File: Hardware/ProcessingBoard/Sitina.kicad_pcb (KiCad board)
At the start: 4 copper layers, 100 x 68 mm, 134 parts, among them J1 Conn_01x30_MountingPin, J200 Conn_02x05_Odd_Even, J500 USB_B_Micro, J700 TXW280064B0, Q400 2N7002, SW200 SW_DIP_x02, SW600 SW_Push, SW601 SW_Push, SW602 SW_Push, SW603 SW_Push, SW610 SW_Push, SW611 SW_Push, SW612 TM-4175-B-B, U100 IMXRT1050, U300 MT48LC16M16A2BG, U400 ADP163, U401 W25Q32JVZP, U500 USBLC6-2SC6, U700 CAT4139, U9 LTC3567, Y100 24MHz, Y101 32.768K

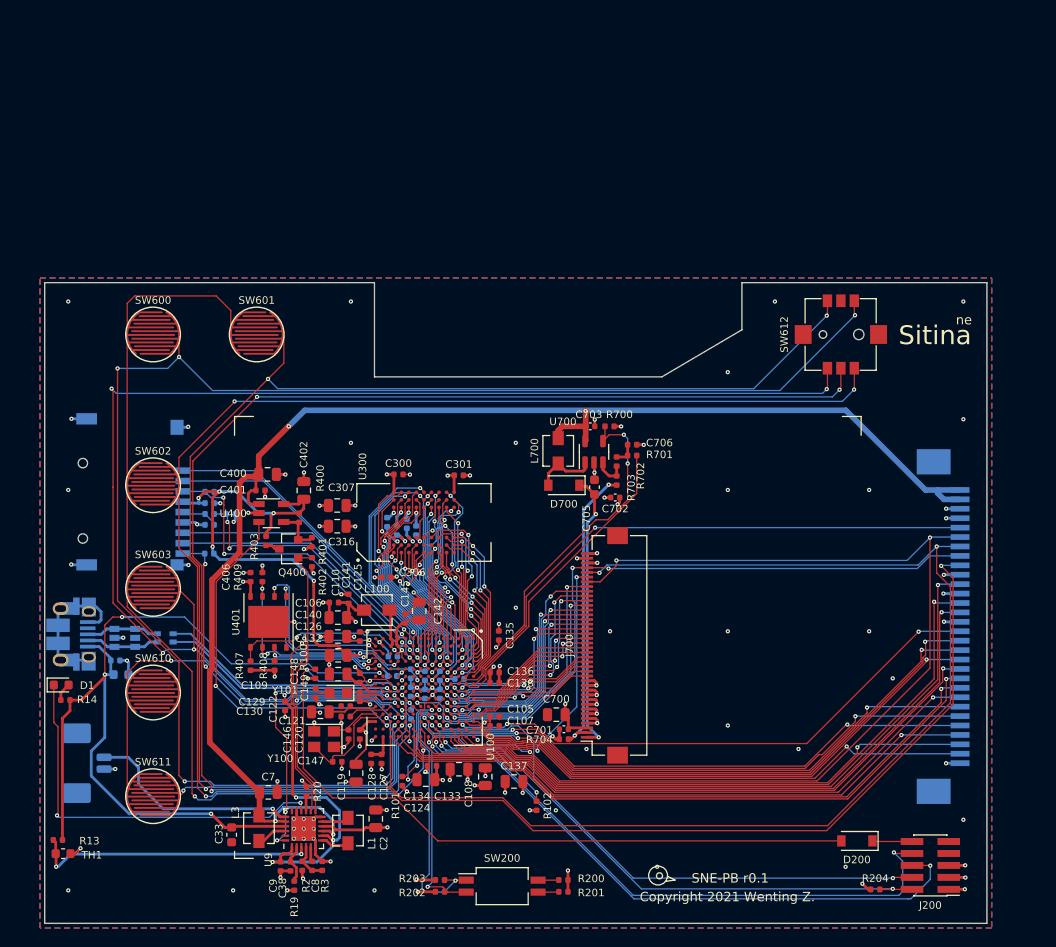
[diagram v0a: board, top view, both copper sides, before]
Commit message: Bug fixes and changes for PB r0p2
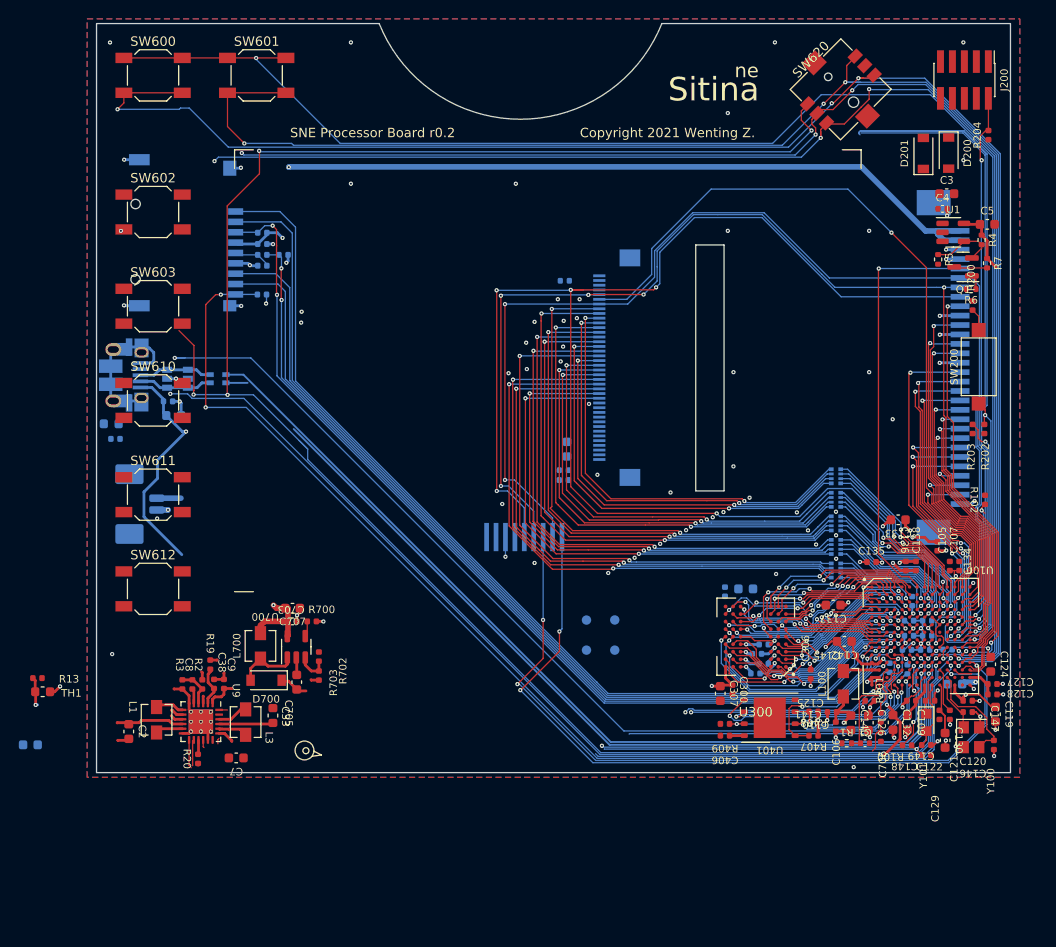
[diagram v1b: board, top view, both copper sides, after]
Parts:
- removed C400: 10uF, Capacitor_SMD:C_0805_2012Metric
- removed C401: 100nF, Capacitor_SMD:C_0402_1005Metric
- removed Q400: 2N7002, Package_TO_SOT_SMD:SOT-23
- removed R101: 10K, Resistor_SMD:R_0402_1005Metric
- removed R201: 1K, Resistor_SMD:R_0402_1005Metric
- removed R400: 464K/1%, Resistor_SMD:R_0402_1005Metric
- removed R401, R402: 200K/1%, Resistor_SMD:R_0402_1005Metric
- removed R403: 243K/1%, Resistor_SMD:R_0402_1005Metric
- removed U400: ADP163, Package_TO_SOT_SMD:TSOT-23-5
- added C1: 0.22uF, Capacitor_SMD:C_0402_1005Metric, F.Cu at (169.6, 139.4)
- added C3: 10uF, Capacitor_SMD:C_0603_1608Metric, F.Cu at (178.2, 81.1)
- added C4: 100nF, Capacitor_SMD:C_0402_1005Metric, F.Cu at (177.8, 82.7)
- added C5: 10uF, Capacitor_SMD:C_0603_1608Metric, F.Cu at (182.5, 84.3)
- added C707: 10uF, Capacitor_SMD:C_0603_1608Metric, F.Cu at (108.8, 125.0)
- added D201: 1N5819, Diode_SMD:D_SOD-123, F.Cu at (175.8, 76.8)
- added J701: Conn_01x09, Footprints:FPC_9, B.Cu at (133.4, 117.5)
- added Q1: 2N7002, Package_TO_SOT_SMD:SOT-23, F.Cu at (180.0, 88.8)
- added R1: 30K, Resistor_SMD:R_0402_1005Metric, F.Cu at (167.6, 139.4)
- added R4: 464K/1%, Resistor_SMD:R_0402_1005Metric, F.Cu at (181.9, 86.0)
- added R5: 200K/1%, Resistor_SMD:R_0402_1005Metric, F.Cu at (177.3, 88.0)
- added R6: 200K/1%, Resistor_SMD:R_0402_1005Metric, F.Cu at (180.8, 91.2)
- added R7: 243K/1%, Resistor_SMD:R_0402_1005Metric, F.Cu at (182.5, 88.4)
- added RN700: 33R, Resistor_SMD:R_Array_Convex_4x0402, B.Cu at (166.5, 111.0)
- added RN701: 33R, Resistor_SMD:R_Array_Convex_4x0402, B.Cu at (166.5, 113.5)
- added RN702: 33R, Resistor_SMD:R_Array_Convex_4x0402, B.Cu at (166.5, 116.0)
- added RN703: 33R, Resistor_SMD:R_Array_Convex_4x0402, B.Cu at (166.5, 118.5)
- added RN704: 33R, Resistor_SMD:R_Array_Convex_4x0402, B.Cu at (166.5, 121.0)
- added SW620: TM-4175-B-B, Footprints:TM4175, F.Cu at (167.0, 70.0)
- added TP1: TestPoint_Small, TestPoint:TestPoint_Pad_D1.0mm, B.Cu at (140.0, 126.3)
- added TP2: TestPoint_Small, TestPoint:TestPoint_Pad_D1.0mm, B.Cu at (140.0, 129.5)
- added TP3: TestPoint_Small, TestPoint:TestPoint_Pad_D1.0mm, B.Cu at (143.0, 126.3)
- added TP4: TestPoint_Small, TestPoint:TestPoint_Pad_D1.0mm, B.Cu at (143.0, 129.5)
- added U1: ADP163, Package_TO_SOT_SMD:TSOT-23-5, F.Cu at (178.9, 85.2)
- C108, C316, C402, C700: footprint Capacitor_SMD:C_0805_2012Metric -> Capacitor_SMD:C_0603_1608Metric; moved to B.Cu
- C109, C119, C124, C126, C130, C132, C133, C137, C140, C142, C2, C307, C7: footprint Capacitor_SMD:C_0805_2012Metric -> Capacitor_SMD:C_0603_1608Metric
- C301, C701, C702, D1, R14, R704: moved to B.Cu
- C404, C405: value 18pF -> DNP
- J700: value TXW280064B0 -> TXW280064B0-R; moved to B.Cu
- L700: value 2.2uH -> 22uH
- SW200: value SW_DIP_x02 -> DNP; footprint Button_Switch_SMD:SW_DIP_SPSTx02_Slide_Copal_CHS-02B_W7.62mm_P1.27mm -> Button_Switch_SMD:SW_SPST_CK_RS282G05A3
- SW600, SW601, SW602, SW603, SW610, SW611: footprint Footprints:contact -> Button_Switch_SMD:SW_SPST_SKQG_WithStem
- SW612: value TM-4175-B-B -> SW_Push; footprint Footprints:TM4175 -> Button_Switch_SMD:SW_SPST_SKQG_WithStem
- U300: footprint Footprints:BGA-54_9x9_8.0x14.0mm -> Footprints:BGA-54_9x9_8.0x8.0mm
- moved J200 83.4 mm to (180.1, 69.0), turned to -90 degrees
- moved R204 81.0 mm to (182.7, 74.8), turned to 90 degrees
- moved SW612 77.8 mm to (94.0, 123.0), turned to 0 degrees
- moved R202 75.8 mm to (182.2, 106.0), turned to -90 degrees
- moved R200 74.9 mm to (181.0, 92.9), turned to 90 degrees
- moved SW200 74.8 mm to (181.6, 99.4), turned to 90 degrees
- moved R203 74.1 mm to (181.0, 106.0), turned to -90 degrees
- moved D200 73.6 mm to (178.4, 76.8), turned to -90 degrees
- moved C147 69.7 mm to (183.2, 139.6), turned to -90 degrees
- moved Y100 68.7 mm to (180.9, 138.8), turned to -90 degrees
- moved C122 68.3 mm to (176.1, 140.6), turned to 0 degrees
- moved C119 68.1 mm to (183.4, 136.3)
- moved C130 66.4 mm to (178.1, 139.1), turned to -90 degrees
- moved C128 66.3 mm to (183.1, 134.2), turned to 0 degrees
- moved C146 65.8 mm to (180.5, 136.1), turned to 0 degrees
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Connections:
- net /MCU/AFE_SYNC renamed /cb_interface/AFE_SYNC
- net /MCU/CSI_D0 renamed /cb_interface/CSI_D0
- net /MCU/CSI_D1 renamed /cb_interface/CSI_D1
- net /MCU/CSI_D10 renamed /cb_interface/CSI_D10
- net /MCU/CSI_D11 renamed /cb_interface/CSI_D11
- net /MCU/CSI_D12 renamed /cb_interface/CSI_D12
- net /MCU/CSI_D13 renamed /cb_interface/CSI_D13
- net /MCU/CSI_D2 renamed /cb_interface/CSI_D2
- net /MCU/CSI_D3 renamed /cb_interface/CSI_D3
- net /MCU/CSI_D4 renamed /cb_interface/CSI_D4
- net /MCU/CSI_D5 renamed /cb_interface/CSI_D5
- net /MCU/CSI_D6 renamed /cb_interface/CSI_D6
- net /MCU/CSI_D7 renamed /cb_interface/CSI_D7
- net /MCU/CSI_D8 renamed /cb_interface/CSI_D8
- net /MCU/CSI_D9 renamed /cb_interface/CSI_D9
- net /MCU/CSI_HSYNC renamed /cb_interface/CSI_HSYNC
- net /MCU/CSI_PCLK renamed /cb_interface/CSI_PCLK
- net /MCU/CSI_VSYNC renamed /cb_interface/CSI_VSYNC
- net /MCU/JTAG_MOD renamed /mcu/JTAG_MOD
- net /MCU/JTAG_TCK renamed /debug/JTAG_TCK
- net /MCU/JTAG_TMS renamed /debug/JTAG_TMS
- net /MCU/KO0 renamed /key/KO0
- net /MCU/LCD_EN renamed /lcd/LCD_EN
- net /MCU/ON renamed /mcu/ON
- net /MCU/POR renamed /debug/SYS_RST
- net /MCU/QSPI_D0 renamed /mcu/QSPI_D0
- net /MCU/QSPI_D1 renamed /mcu/QSPI_D1
- net /MCU/QSPI_D2 renamed /mcu/QSPI_D2
- net /MCU/QSPI_D3 renamed /mcu/QSPI_D3
- net /MCU/QSPI_SCK renamed /mcu/QSPI_SCK
- net /MCU/QSPI_SS_B renamed /mcu/QSPI_SS_B
- net /MCU/SDRAM_A0 renamed /mcu/SDRAM_A0
- net /MCU/SDRAM_A1 renamed /mcu/SDRAM_A1
- net /MCU/SDRAM_A10 renamed /mcu/SDRAM_A10
- net /MCU/SDRAM_A11 renamed /mcu/SDRAM_A11
- net /MCU/SDRAM_A12 renamed /mcu/SDRAM_A12
- net /MCU/SDRAM_A2 renamed /mcu/SDRAM_A2
- net /MCU/SDRAM_A3 renamed /mcu/SDRAM_A3
- net /MCU/SDRAM_A4 renamed /mcu/SDRAM_A4
- net /MCU/SDRAM_A5 renamed /mcu/SDRAM_A5
- net /MCU/SDRAM_A6 renamed /mcu/SDRAM_A6
- net /MCU/SDRAM_A7 renamed /mcu/SDRAM_A7
- net /MCU/SDRAM_A8 renamed /mcu/SDRAM_A8
- net /MCU/SDRAM_A9 renamed /mcu/SDRAM_A9
- net /MCU/SDRAM_BA0 renamed /mcu/SDRAM_BA0
- net /MCU/SDRAM_BA1 renamed /mcu/SDRAM_BA1
- net /MCU/SDRAM_CKE renamed /sdram/SDRAM_CKE
- net /MCU/SDRAM_CLK renamed /sdram/SDRAM_CLK
- net /MCU/SDRAM_D0 renamed /mcu/SDRAM_D0
- net /MCU/SDRAM_D1 renamed /mcu/SDRAM_D1
- net /MCU/SDRAM_D10 renamed /mcu/SDRAM_D10
- net /MCU/SDRAM_D11 renamed /mcu/SDRAM_D11
- net /MCU/SDRAM_D12 renamed /mcu/SDRAM_D12
- net /MCU/SDRAM_D13 renamed /mcu/SDRAM_D13
- net /MCU/SDRAM_D14 renamed /mcu/SDRAM_D14
- net /MCU/SDRAM_D15 renamed /mcu/SDRAM_D15
- net /MCU/SDRAM_D2 renamed /mcu/SDRAM_D2
- net /MCU/SDRAM_D3 renamed /mcu/SDRAM_D3
- net /MCU/SDRAM_D4 renamed /mcu/SDRAM_D4
- net /MCU/SDRAM_D5 renamed /mcu/SDRAM_D5
- net /MCU/SDRAM_D6 renamed /mcu/SDRAM_D6
- net /MCU/SDRAM_D7 renamed /mcu/SDRAM_D7
- net /MCU/SDRAM_D8 renamed /mcu/SDRAM_D8
- net /MCU/SDRAM_D9 renamed /mcu/SDRAM_D9
- net /MCU/SDRAM_DM0 renamed /mcu/SDRAM_DM0
- net /MCU/SDRAM_DM1 renamed /mcu/SDRAM_DM1
- net /MCU/SD_CD_B renamed /mcu/SD_CD_B
- net /MCU/SD_CLK renamed /mcu/SD_CLK
- net /MCU/SD_D0 renamed /mcu/SD_D0
- net /MCU/SD_D1 renamed /mcu/SD_D1
- net /MCU/SD_D2 renamed /mcu/SD_D2
- net /MCU/SD_D3 renamed /mcu/SD_D3
- net /MCU/USB_DP renamed /mcu/USB_DP
- net /SDRAM/SDRAM_CAS renamed /sdram/SDRAM_CAS
- net /SDRAM/SDRAM_CS0 renamed /sdram/SDRAM_CS0
- net /SDRAM/SDRAM_RAS renamed /sdram/SDRAM_RAS
- net /SDRAM/SDRAM_WE renamed /sdram/SDRAM_WE
- net /storage/SD_CMD renamed /mcu/SD_CMD
- net /usb/USB_DM renamed /mcu/USB_DN
- C402 pad 1: +VSD -> +3V3
- C403 pad 1: +VSD -> +3V3
- J1 pad 22: /MCU/SPI_CS -> /cb_interface/AFE_SL
- J1 pad 23: /MCU/LCD_DI -> /cb_interface/AFE_SDATA
- J1 pad 24: /MCU/LCD_SCK -> /cb_interface/AFE_SCK
- J1 pad 25: /connector/AFE_RST -> /cb_interface/AFE_RST
- J200 pad 1: +3V3 -> Net-(D201-Pad2)
- J200 pad 6: /MCU/JTAG_TDO -> (no net)
- J200 pad 8: /MCU/JTAG_TDI -> (no net)
- J700 pad 1: /lcd/LEDA -> GND
- J700 pad 10: GND -> /lcd/D_D13
- J700 pad 11: GND -> /lcd/D_D12
- J700 pad 12: GND -> /lcd/D_D11
- J700 pad 13: GND -> /lcd/D_D10
- J700 pad 14: /MCU/LCD_VSYNC -> /lcd/D_D9
- J700 pad 15: /MCU/LCD_HSYNC -> /lcd/D_D8
- J700 pad 16: /MCU/LCD_CLK -> /lcd/D_D7
- J700 pad 17: /MCU/LCD_DE -> /lcd/D_D6
- J700 pad 18: /MCU/LCD_D0 -> /lcd/D_D5
- J700 pad 19: /MCU/LCD_D1 -> /lcd/D_D4
- J700 pad 2: /lcd/LEDK -> +3V3
- J700 pad 20: /MCU/LCD_D2 -> /lcd/D_D3
- J700 pad 21: /MCU/LCD_D3 -> /lcd/D_D2
- J700 pad 22: /MCU/LCD_D4 -> /lcd/D_D1
- J700 pad 23: /MCU/LCD_D5 -> /lcd/D_D0
- J700 pad 24: /MCU/LCD_D6 -> /lcd/D_DE
- J700 pad 25: /MCU/LCD_D7 -> /lcd/D_DCLK
- J700 pad 26: /MCU/LCD_D8 -> /lcd/D_HSYNC
- J700 pad 27: /MCU/LCD_D9 -> /lcd/D_VSYNC
- J700 pad 28: /MCU/LCD_D10 -> GND
- J700 pad 29: /MCU/LCD_D11 -> GND
- J700 pad 3: +3V3 -> GND
- J700 pad 30: /MCU/LCD_D12 -> GND
- J700 pad 31: /MCU/LCD_D13 -> GND
- J700 pad 32: /MCU/LCD_D14 -> GND
- J700 pad 33: /MCU/LCD_D15 -> GND
- J700 pad 34: /connector/AFE_RST -> GND
- J700 pad 35: /MCU/LCD_CS -> GND
- J700 pad 36: /MCU/LCD_SCK -> GND
- J700 pad 37: /MCU/LCD_DI -> GND
- J700 pad 38: GND -> +3V3
- J700 pad 39: +3V3 -> /lcd/LEDK
- J700 pad 4: GND -> /cb_interface/AFE_SDATA
- J700 pad 40: GND -> /lcd/LEDA
- J700 pad 5: GND -> /cb_interface/AFE_SCK
- J700 pad 6: GND -> /lcd/LCD_CSN
- J700 pad 7: GND -> /cb_interface/AFE_RST
- J700 pad 8: GND -> /lcd/D_D15
- J700 pad 9: GND -> /lcd/D_D14
- MICRO_SD400 pad 4: +VSD -> +3V3
- R100 pad 1: +3V3 -> +VRTC
- R13 pad 1: Net-(R13-Pad1) -> VBUS
- R202 pad 1: /MCU/BOOT0 -> /debug/BOOT0
- R203 pad 1: /MCU/BOOT1 -> /debug/BOOT1
- R405 pad 1: +VSD -> +3V3
- R406 pad 1: +VSD -> +3V3
- R701 pad 2: /MCU/LCD_PWM -> /lcd/LCD_PWM
- SW200 pad 1: /MCU/BOOT1 -> /debug/BOOT0
- SW200 pad 2: /MCU/BOOT0 -> Net-(R200-Pad1)
- SW600 pad 2: /MCU/KI0 -> /key/KI0
- SW601 pad 2: /MCU/KI1 -> /key/KI1
- SW602 pad 2: /MCU/KI2 -> /key/KI2
- SW603 pad 2: /MCU/KI3 -> /key/KI3
- SW610 pad 1: /MCU/KO1 -> /key/KO1
- SW610 pad 2: /MCU/KI0 -> /key/KI0
- SW611 pad 1: /MCU/KO1 -> /key/KO1
- SW611 pad 2: /MCU/KI1 -> /key/KI1
- SW612 pad 1: /MCU/KI0 -> /key/KO1
- SW612 pad 2: (no net) -> /key/KI2
- TH1 pad 1: Net-(R13-Pad1) -> VBUS
- U100 pad A10: /MCU/LCD_D7 -> /lcd/LCD_D7
- U100 pad A11: /MCU/LCD_D12 -> /lcd/LCD_D12
- U100 pad A8: /MCU/LCD_D2 -> /lcd/LCD_D2
- U100 pad A9: /MCU/LCD_D3 -> /lcd/LCD_D3
- U100 pad B11: /MCU/LCD_D13 -> /lcd/LCD_D13
- U100 pad B14: /MCU/LCD_CS -> /lcd/LCD_CSN
- U100 pad B7: /MCU/LCD_PWM -> (no net)
- U100 pad B8: /MCU/LCD_D1 -> /lcd/LCD_D1
- U100 pad B9: /MCU/LCD_D4 -> /lcd/LCD_D4
- U100 pad C10: /MCU/LCD_D8 -> /lcd/LCD_D8
- U100 pad C11: /MCU/LCD_D14 -> /lcd/LCD_D14
- U100 pad C8: /MCU/LCD_D0 -> /lcd/LCD_D0
- U100 pad C9: /MCU/LCD_D5 -> /lcd/LCD_D5
- U100 pad D10: /MCU/LCD_D9 -> /lcd/LCD_D9
- U100 pad D11: /MCU/LCD_D15 -> /lcd/LCD_D15
- U100 pad D7: /MCU/LCD_CLK -> /lcd/LCD_CLK
- U100 pad D8: /MCU/LCD_VSYNC -> /lcd/LCD_VSYNC
- U100 pad D9: /MCU/LCD_D6 -> /lcd/LCD_D6
- U100 pad E10: /MCU/LCD_D10 -> /lcd/LCD_D10
- U100 pad E11: /MCU/LCD_D11 -> /lcd/LCD_D11
- U100 pad E7: /MCU/LCD_DE -> /lcd/LCD_DE
- U100 pad E8: /MCU/LCD_HSYNC -> /lcd/LCD_HSYNC
- U100 pad F11: /MCU/BOOT1 -> /debug/BOOT0
- U100 pad F14: /MCU/JTAG_TDI -> /grip_interface/USER1
- U100 pad G10: /MCU/JTAG_TRSTB -> (no net)
- U100 pad G11: /MCU/BOOT0 -> /cb_interface/AFE_RST
- U100 pad G13: /MCU/JTAG_TDO -> /grip_interface/USER2
- U100 pad G14: /connector/AFE_RST -> /debug/BOOT1
- U100 pad H10: /MCU/LCD_DI -> /cb_interface/AFE_SDATA
- U100 pad J11: /MCU/KO2 -> /key/KO2
- U100 pad J12: /MCU/KI2 -> /key/KI2
- U100 pad K10: /MCU/KI3 -> /key/KI3
- U100 pad K11: /MCU/SD_VSELECT -> /mcu/SD_VSELECT
- U100 pad K12: /MCU/KI1 -> /key/KI1
- U100 pad K14: (no net) -> /cb_interface/AFE_SL
- U100 pad K3: +3V3 -> Net-(C1-Pad1)
- U100 pad L10: /MCU/KO1 -> /key/KO1
- U100 pad L12: /MCU/KI0 -> /key/KI0
- U100 pad L14: (no net) -> /lcd/LCD2_CS
- U100 pad M11: /MCU/SPI_CS -> /lcd/LCD2_RS
- U100 pad M12: /MCU/SD_PWR_EN -> /grip_interface/SHUTTER
- U100 pad M14: /MCU/LCD_SCK -> /cb_interface/AFE_SCK
- U100 pad M3: (no net) -> /mcu/I2C_SCL
- U100 pad M5: (no net) -> /lcd/LCD_PWM
- U100 pad M6: (no net) -> /grip_interface/ONOFF
- U100 pad N3: /MCU/I2C_SDA -> (no net)
- U100 pad P2: /MCU/I2C_SCL -> /mcu/I2C_SDA
- U9 pad 13: /MCU/I2C_SCL -> /mcu/I2C_SCL
- U9 pad 14: /MCU/I2C_SDA -> /mcu/I2C_SDA
- U9 pad 3: Net-(R13-Pad1) -> VBUS
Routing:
- net /key/KI3: track 0.00 -> 203.8 mm, vias 0 -> 5
- net /key/KI0: track 0.00 -> 170.5 mm, vias 0 -> 4
- net /cb_interface/AFE_SDATA: track 0.00 -> 168.3 mm, vias 0 -> 6
- net /MCU/KI0: track 163.3 -> 0.00 mm, vias 5 -> 0
- net /key/KI1: track 0.00 -> 161.1 mm, vias 0 -> 5
- net /MCU/KI1: track 148.5 -> 0.00 mm, vias 5 -> 0
- net /key/KO2: track 0.00 -> 148.3 mm, vias 0 -> 4
- net /key/KI2: track 0.00 -> 148.0 mm, vias 0 -> 4
- net /MCU/KI3: track 144.7 -> 0.00 mm, vias 5 -> 0
- net /MCU/KI2: track 142.9 -> 0.00 mm, vias 4 -> 0
- net /MCU/KO2: track 139.8 -> 0.00 mm, vias 4 -> 0
- net /cb_interface/AFE_SCK: track 0.00 -> 131.0 mm, vias 0 -> 5
- net /MCU/LCD_SCK: track 129.8 -> 0.00 mm, vias 2 -> 0
- net /cb_interface/AFE_RST: track 0.00 -> 129.1 mm, vias 0 -> 3
- net /connector/AFE_RST: track 116.7 -> 0.00 mm, vias 4 -> 0
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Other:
- board size 100 x 68 mm -> 97 x 79.5 mm
- board text added: "SNE Processor Board r0.2"
- board text removed: "SNE-PB r0.1"
